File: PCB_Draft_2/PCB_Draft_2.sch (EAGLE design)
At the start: 23 parts, among them SW1 PUSHBUTTON, SW2 PUSHBUTTON

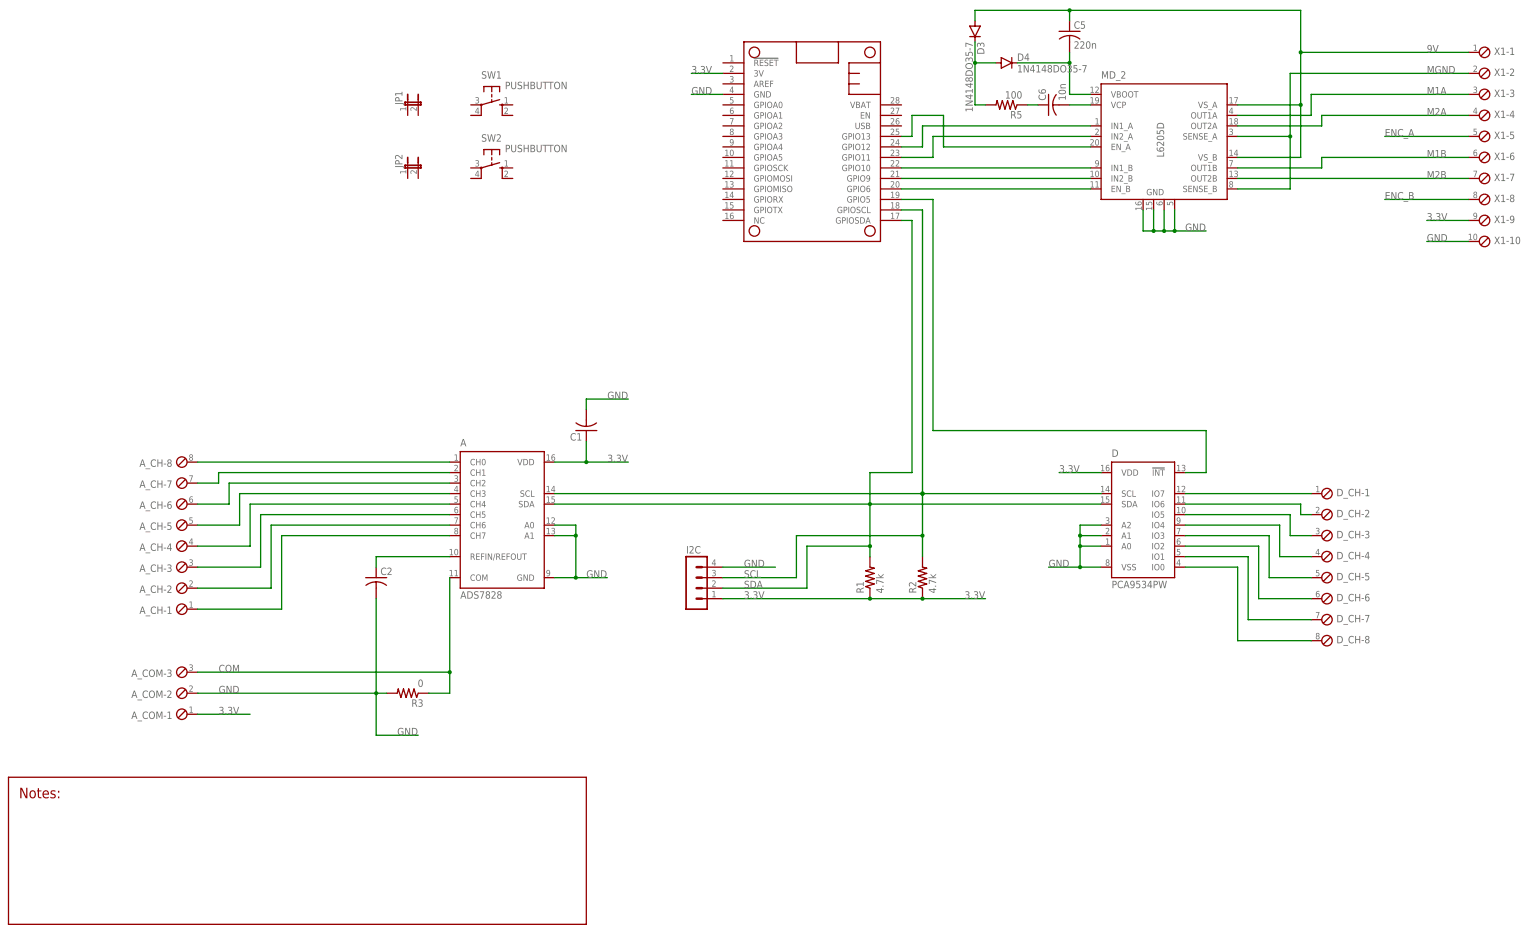
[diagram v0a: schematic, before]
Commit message: Near-final draft - all wires run; checking formatting
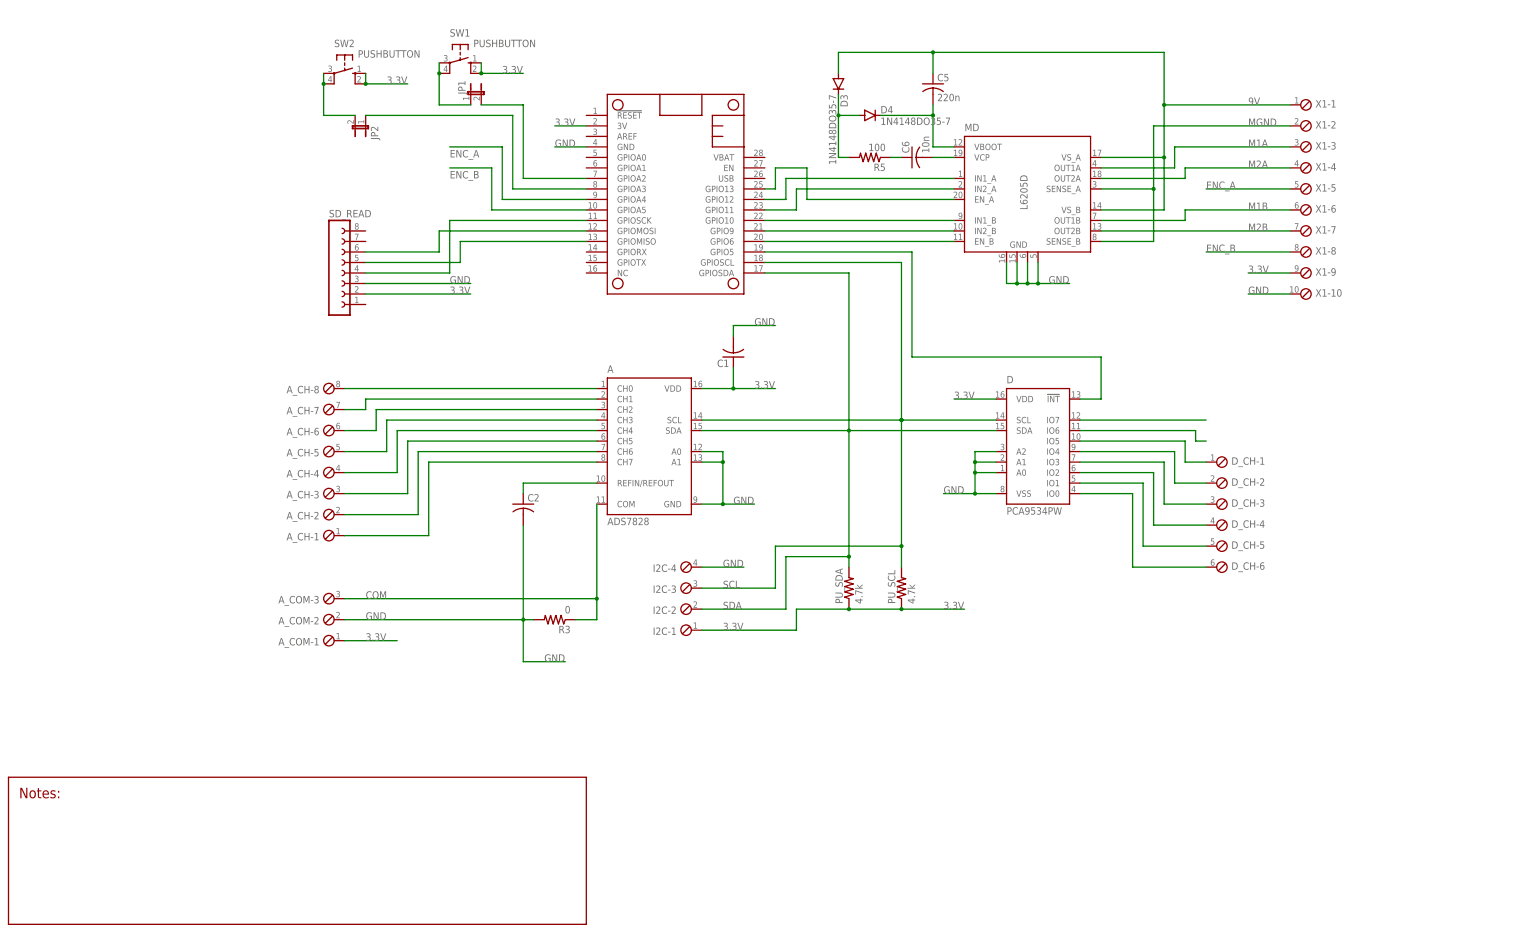
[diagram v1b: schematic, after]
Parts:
- removed MD_2: L6205D, st-microelectronics:L6205D
- removed R1, R2: 4.7k, rcl:R-US_M0805
- added MD: L6205D, st-microelectronics:L6205D
- added PU_SCL, PU_SDA: 4.7k, rcl:R-US_M0805
- added SD_READ: (no value), con-lsta:FE08-1
- D_CH: device ME507:SCREWTERM_8P_254 -> ME507:SCREWTERM_6P_254
- I2C: device con-lstb:MA04-1 -> ME507:SCREWTERM_4P_254
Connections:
- new net N$24: FTHRWNG.GPIOSCK, SD_READ.4
- new net N$26: JP1.1, SW1.P, SW1.P1
- new net N$27: JP2.2, SW2.P, SW2.P1
- new net N$28: FTHRWNG.GPIOMISO, SD_READ.5
- new net N$29: FTHRWNG.GPIOA3, JP2.1
- new net N$30: FTHRWNG.GPIOA2, JP1.2
- new net N$31: FTHRWNG.GPIOMOSI, SD_READ.6
- net 3.3V: now also I2C-1.1, PU_SCL.1, PU_SDA.1, SD_READ.2, SW1.S, SW1.S1, SW2.S, SW2.S1; no longer I2C.1, R1.1, R2.1
- net 9V: now also MD.VS_A, MD.VS_B; no longer MD_2.VS_A, MD_2.VS_B
- net ENC_A: now also FTHRWNG.GPIOA4
- net ENC_B: now also FTHRWNG.GPIOA5
- net GND: now also I2C-4.1, MD.GND, MD.GND@1, MD.GND@2, MD.GND@3, SD_READ.3; no longer I2C.4, MD_2.GND, MD_2.GND@1, MD_2.GND@2, MD_2.GND@3
- net M1A: now also MD.OUT1A; no longer MD_2.OUT1A
- net M1B: now also MD.OUT1B; no longer MD_2.OUT1B
- net M2A: now also MD.OUT2A; no longer MD_2.OUT2A
- net M2B: now also MD.OUT2B; no longer MD_2.OUT2B
- net MGND: now also MD.SENSE_A, MD.SENSE_B; no longer MD_2.SENSE_A, MD_2.SENSE_B
- net N$1: no longer D_CH-1.1
- net N$18: now also MD.EN_B; no longer MD_2.EN_B
- net N$2: no longer D_CH-2.1
- net N$20: now also MD.IN2_B; no longer MD_2.IN2_B
- net N$21: now also MD.IN1_B; no longer MD_2.IN1_B
- net N$22: now also MD.IN2_A; no longer MD_2.IN2_A
- net N$23: now also MD.IN1_A; no longer MD_2.IN1_A
- net N$25: now also MD.EN_A; no longer MD_2.EN_A
- net N$3: now also D_CH-1.1; no longer D_CH-3.1
- net N$4: now also D_CH-2.1; no longer D_CH-4.1
- net N$43: now also MD.VCP; no longer MD_2.VCP
- net N$46: now also MD.VBOOT; no longer MD_2.VBOOT
- net N$5: now also D_CH-3.1; no longer D_CH-5.1
- net N$6: now also D_CH-4.1; no longer D_CH-6.1
- net N$7: now also D_CH-5.1; no longer D_CH-7.1
- net N$8: now also D_CH-6.1; no longer D_CH-8.1
- net SCL: now also I2C-3.1, PU_SCL.2; no longer I2C.3, R2.2
- net SDA: now also I2C-2.1, PU_SDA.2; no longer I2C.2, R1.2
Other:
- moved on the sheet: A, A_CH-1, A_CH-2, A_CH-3, A_CH-4, A_CH-5, A_CH-6, A_CH-7, A_CH-8, A_COM-1, A_COM-2, A_COM-3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
